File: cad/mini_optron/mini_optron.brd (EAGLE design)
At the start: 67 x 39.4 mm, 10 parts

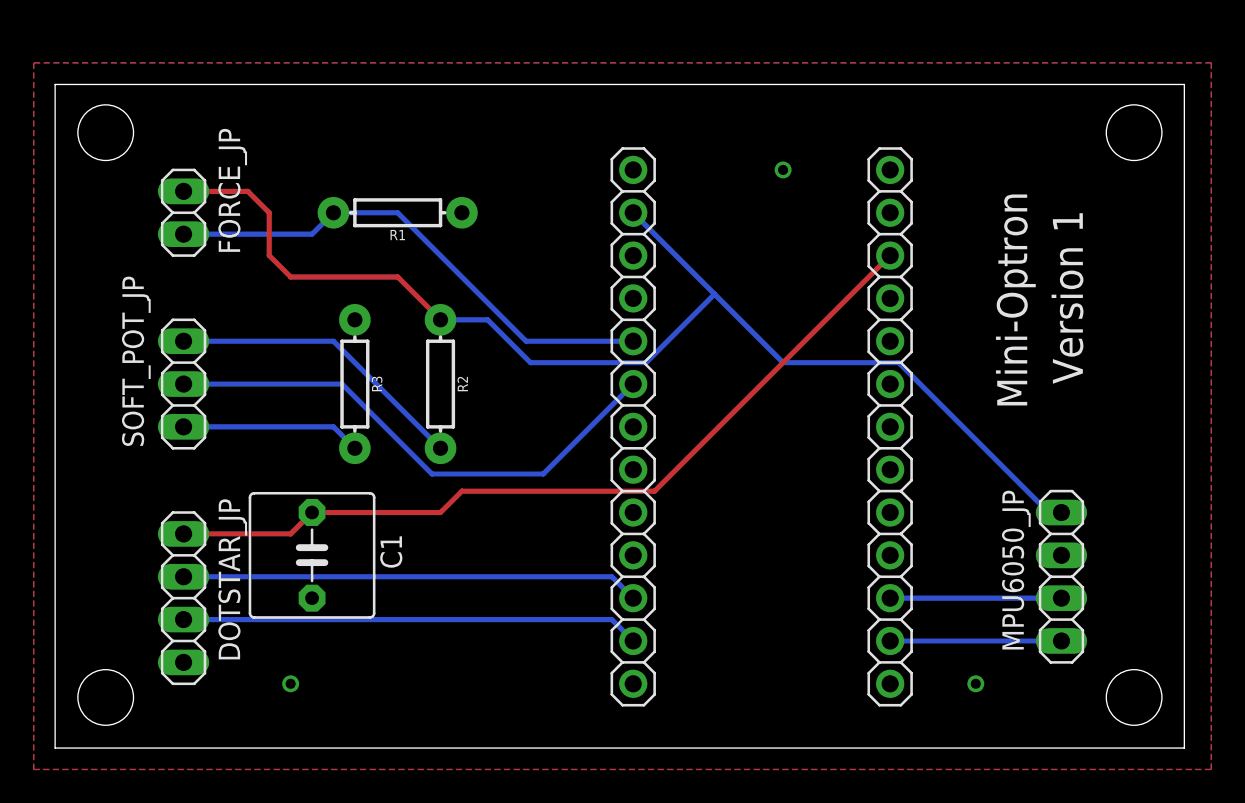
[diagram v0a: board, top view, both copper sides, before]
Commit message: Add files via upload
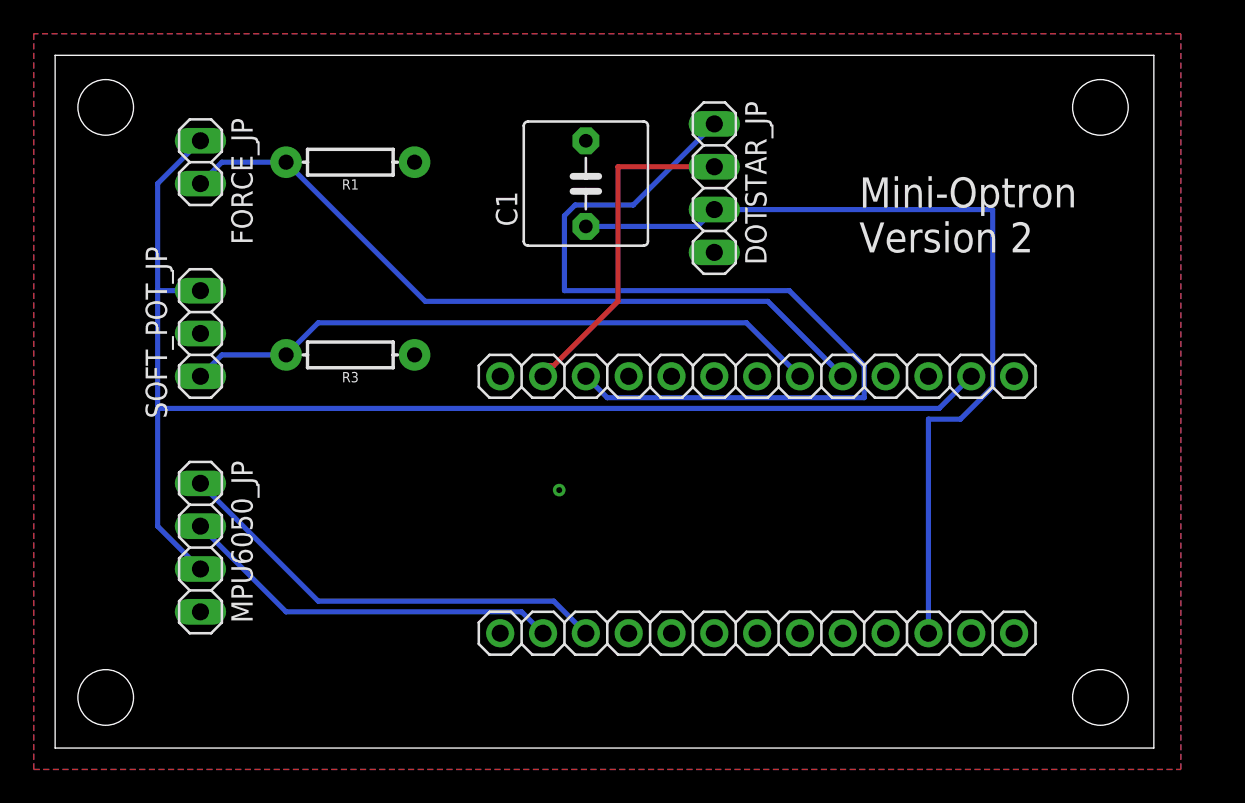
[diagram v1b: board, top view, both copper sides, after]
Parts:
- removed R2: 10k, SparkFun-Resistors:AXIAL-0.3
- R1: value 33k -> 10K
- moved MPU6050_JP 51.1 mm to (8.62, 11.9)
- moved DOTSTAR_JP 39.8 mm to (39.1, 33.2)
- moved C1 27.4 mm to (31.5, 33.5), turned to 90 degrees
- moved JP2 14.6 mm to (41.6, 6.81), turned to 180 degrees
- moved JP1 7.94 mm to (41.6, 22.1), turned to 180 degrees
- moved R1 4.11 mm to (17.5, 34.8)
- moved FORCE_JP 3.16 mm to (8.62, 34.8)
- moved SOFT_POT_JP 3.16 mm to (8.62, 24.6)
- moved R3 1.75 mm to (17.5, 23.3), turned to 180 degrees
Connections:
- net N$1 renamed A0
- removed net CONN: FORCE_JP.1, JP1.2, MPU6050_JP.1, R2.P$1
- removed net N$10: JP2.12, MPU6050_JP.4
- removed net N$2: DOTSTAR_JP.2, JP1.11
- removed net N$3: R2.P$2, SOFT_POT_JP.1
- removed net N$4: JP1.6, SOFT_POT_JP.2
- removed net N$5: R3.P$2, SOFT_POT_JP.3
- removed net N$6: DOTSTAR_JP.3, JP1.12
- removed net N$9: JP2.11, MPU6050_JP.3
- removed net VCC: C1.1, DOTSTAR_JP.1, JP2.3
- new net 3V: FORCE_JP.1, JP1.2, MPU6050_JP.3, SOFT_POT_JP.1
- new net 5V: C1.1, DOTSTAR_JP.3, JP2.3
- new net A1: JP1.6, R3.P$2, SOFT_POT_JP.3
- new net MOSI: DOTSTAR_JP.2, JP1.12
- new net SCK: DOTSTAR_JP.1, JP1.11
- new net SCL: JP2.11, MPU6050_JP.1
- new net SDA: JP2.12, MPU6050_JP.2
- net GND: now also MPU6050_JP.4, SOFT_POT_JP.2; no longer MPU6050_JP.2
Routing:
- net 3V: track 0.00 -> 79.1 mm
- net CONN: track 71.6 -> 0.00 mm
- net SCK: track 0.00 -> 54.2 mm
- net 5V: track 0.00 -> 52.4 mm
- net VCC: track 48.7 -> 0.00 mm
- net A1: track 0.00 -> 38.2 mm
- net N$4: track 31.1 -> 0.00 mm
- net N$6: track 27.2 -> 0.00 mm
- net N$2: track 27.2 -> 0.00 mm
- net SCL: track 0.00 -> 26.5 mm
- net SDA: track 0.00 -> 23.0 mm
- net MOSI: track 0.00 -> 20.4 mm
- net N$3: track 17.9 -> 0.00 mm
- net A0: track 30.4 -> 43.9 mm
- net N$5: track 10.7 -> 0.00 mm
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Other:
- board size 67 x 39.4 mm -> 65.2 x 41.1 mm
- board text added: "Mini-Optron Version 2"
- board text removed: "Mini-Optron"
- board text removed: "Version 1"
